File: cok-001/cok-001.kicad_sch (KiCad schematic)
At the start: 72 parts, among them J3209 ATA Power, J3221 ATA0 for BD, U2101 ADT7461A0002RMZR, U2105 TC7WP3125FK, U2108 ICS651MLFT, U6005 NCP511SN33T1G, U6006 NCP511SN18T1, U6009 NCP511SN33T1G, Y2101 24.576MHz

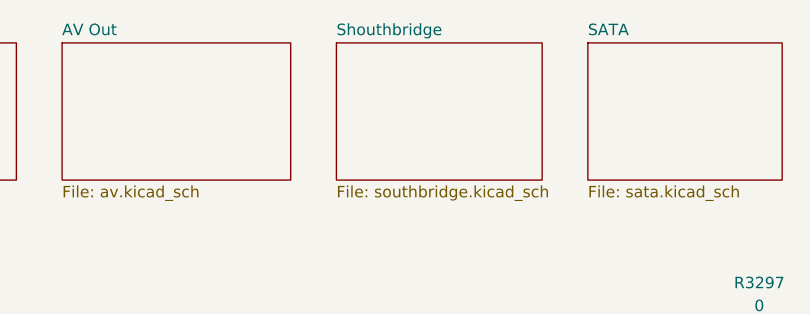
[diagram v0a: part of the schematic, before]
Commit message: L
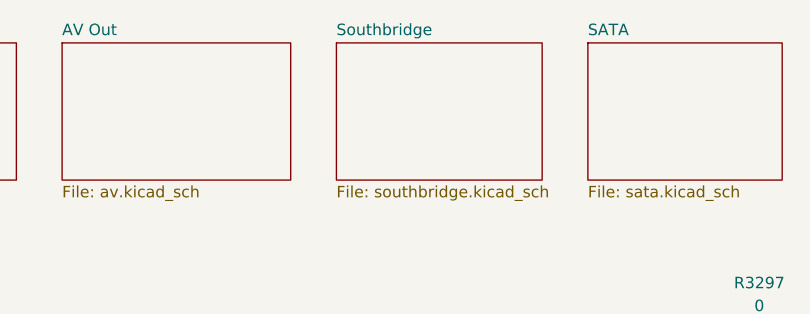
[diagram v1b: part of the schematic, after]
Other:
- sheet Shouthbridge renamed Southbridge
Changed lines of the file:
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@@
 			(color 0 0 0 0.0000)
 		)
-		(property "Sheetname" "Shouthbridge"
+		(property "Sheetname" "Southbridge"
 			(at 364.49 13.2584 0)
 			(effects
@@
 			(project "cok-001"
 				(path "/976eb78d-8215-4cc0-9d72-f9d535c7970b"
-					(page "13")
+					(page "30")
 				)
 			)

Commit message: seperate out
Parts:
- removed C2101, C2102, C2125: XX, Capacitor_SMD:C_0402_1005Metric, symbol Device:C
- removed C2103: 0.001u 50V, Capacitor_SMD:C_0402_1005Metric, symbol Device:C
- removed C2108: 0.1u 10V, Capacitor_SMD:C_0402_1005Metric, symbol Device:C
- removed C2109: 8p, Capacitor_SMD:C_0402_1005Metric, symbol Device:C
- removed C2112: 9p, Capacitor_SMD:C_0402_1005Metric, symbol Device:C
- removed C2271: 0.01u 25V, Capacitor_SMD:C_0402_1005Metric, symbol Device:C
- removed C2272: 100p, Capacitor_SMD:C_0402_1005Metric, symbol Device:C
- removed C3246: 47u 25V, Capacitor_Tantalum_SMD:CP_EIA-3528-15_AVX-H, symbol Device:C_Polarized_US
- removed C3247: 47u 25V, Capacitor_Tantalum_SMD:CP_EIA-7132-28_AVX-C, symbol Device:C_Polarized_US
- removed D3208: LED_Dual_AAKK, Package_TO_SOT_SMD:SC-82AA, symbol Device:LED_Dual_AAKK
- removed F6302: 5A, Fuse:Fuse_1206_3216Metric, symbol Device:Fuse
- removed J3209: ATA Power, Connector_JST:JST_PH_B4B-PH-SM4-TB_1x04-1MP_P2.00mm_Vertical, symbol Connector:Conn_01x04_Socket
- removed J3221: ATA0 for BD, PS3:Hirose_FH12-60S, symbol Connector:Conn_01x60_Pin
- removed L6302: 1uH, Inductor_SMD:L_TDK_SLF6028, symbol Device:L
- removed R2101, R2102: 100, Resistor_SMD:R_0402_1005Metric, symbol Device:R_US
- removed R2103, R2104, R2117: 43,2, Resistor_SMD:R_0402_1005Metric, symbol Device:R_US
- removed R2106: 10k, Resistor_SMD:R_0402_1005Metric, symbol Device:R_US
- removed R2107: 0, Resistor_SMD:R_0603_1608Metric, symbol Device:R_US
- removed R2109: 39, Resistor_SMD:R_0402_1005Metric, symbol Device:R_US
- removed R2123, R2177, R2179: 33, Resistor_SMD:R_0402_1005Metric, symbol Device:R_US
- removed R2181: R, Resistor_SMD:R_0402_1005Metric, symbol Device:R_US
- removed R3211, R3225, R3226, R3227: 0, Resistor_SMD:R_0402_1005Metric, symbol Device:R_US
- removed R3297: 0, Resistor_SMD:R_0805_2012Metric, symbol Device:R_US
- removed U2101: ADT7461A0002RMZR, Package_SO:MSOP-8_3x3mm_P0.65mm, symbol PS3:ADT7461A
- removed U2102: ~, Package_SO:SSOP-24_3.9x8.7mm_P0.635mm, symbol PS3:ICS422A
- removed U2105: TC7WP3125FK, Package_SO:VSSOP-8_2.3x2mm_P0.5mm, symbol PS3:TC7WP3125FK
- removed U2108: ICS651MLFT, Package_SO:SOIC-8_3.9x4.9mm_P1.27mm, symbol PS3:ICS651
- removed Y2101: 24.576MHz, Crystal:Crystal_SMD_5032-2Pin_5.0x3.2mm, symbol Device:Crystal
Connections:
- no-connect marks 3 -> 0
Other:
- added sheet External (external.kicad_sch)
- added sheet RSX Setting (rsxsetting.kicad_sch)
- added sheet SB MISC (sbmisc.kicad_sch)
- added sheet VRM for RSX (rsxvrm.kicad_sch)
- moved on the sheet: C5064, C5070, C5153, C6116, C6117, C6118, C6217, C6218, H1, H10, H11, H12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

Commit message: update to 9
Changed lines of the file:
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@@
 (kicad_sch
-	(version 20231120)
+	(version 20250114)
 	(generator "eeschema")
-	(generator_version "8.0")
+	(generator_version "9.0")
 	(paper "A4")
 	(junction
@@
 		(at 363.22 15.24)
 		(size 25.4 15.24)
+		(exclude_from_sim no)
+		(in_bom yes)
+		(on_board yes)
+		(dnp no)
 		(fields_autoplaced yes)
 		(stroke
@@
 		(at 76.2 15.24)
 		(size 25.4 15.24)
+		(exclude_from_sim no)
+		(in_bom yes)
+		(on_board yes)
+		(dnp no)
 		(fields_autoplaced yes)
 		(stroke
@@
 		(at 15.24 38.1)
 		(size 22.86 15.24)
+		(exclude_from_sim no)
+		(in_bom yes)
+		(on_board yes)
+		(dnp no)
 		(fields_autoplaced yes)
 		(stroke
@@
 		(at 332.74 15.24)
 		(size 25.4 15.24)
+		(exclude_from_sim no)
+		(in_bom yes)
+		(on_board yes)
+		(dnp no)
 		(fields_autoplaced yes)
 		(stroke
@@
 		(at 302.26 38.1)
 		(size 27.94 15.24)
+		(exclude_from_sim no)
+		(in_bom yes)
+		(on_board yes)
+		(dnp no)
 		(fields_autoplaced yes)
 		(stroke
@@
 		(at 110.49 15.24)
 		(size 26.67 15.24)
+		(exclude_from_sim no)
+		(in_bom yes)
+		(on_board yes)
+		(dnp no)
 		(fields_autoplaced yes)
 		(stroke
@@
 		(at 144.78 15.24)
 		(size 25.4 15.24)
+		(exclude_from_sim no)
+		(in_bom yes)
+		(on_board yes)
+		(dnp no)
 		(fields_autoplaced yes)
 		(stroke
@@
 		(at 209.55 15.24)
 		(size 24.13 15.24)
+		(exclude_from_sim no)
+		(in_bom yes)
+		(on_board yes)
+		(dnp no)
 		(fields_autoplaced yes)
 		(stroke
@@
 		(at 177.8 15.24)
 		(size 25.4 15.24)
+		(exclude_from_sim no)
+		(in_bom yes)
+		(on_board yes)
+		(dnp no)
 		(fields_autoplaced yes)
 		(stroke
@@
 		(at 419.1 15.24)
 		(size 25.4 15.24)
+		(exclude_from_sim no)
+		(in_bom yes)
+		(on_board yes)
+		(dnp no)
 		(fields_autoplaced yes)
 		(stroke
@@
 		(at 269.24 15.24)
 		(size 25.4 15.24)
+		(exclude_from_sim no)
+		(in_bom yes)
+		(on_board yes)
+		(dnp no)
 		(fields_autoplaced yes)
 		(stroke
@@
 		(at 238.76 15.24)
 		(size 25.4 15.24)
+		(exclude_from_sim no)
+		(in_bom yes)
+		(on_board yes)
+		(dnp no)
 		(fields_autoplaced yes)
 		(stroke
@@
 		(at 45.72 15.24)
 		(size 22.86 15.24)
+		(exclude_from_sim no)
+		(in_bom yes)
+		(on_board yes)
+		(dnp no)
 		(fields_autoplaced yes)
 		(stroke
@@
 		(at 302.26 15.24)
 		(size 25.4 15.24)
+		(exclude_from_sim no)
+		(in_bom yes)
+		(on_board yes)
+		(dnp no)
 		(fields_autoplaced yes)
 		(stroke
@@
 		(at 332.74 38.1)
 		(size 25.4 15.24)
+		(exclude_from_sim no)
+		(in_bom yes)
+		(on_board yes)
+		(dnp no)
 		(fields_autoplaced yes)
 		(stroke
@@
 		(at 15.24 15.24)
 		(size 22.86 15.24)
+		(exclude_from_sim no)
+		(in_bom yes)
+		(on_board yes)
+		(dnp no)
 		(fields_autoplaced yes)
 		(stroke
@@
 		(at 363.22 38.1)
 		(size 25.4 15.24)
+		(exclude_from_sim no)
+		(in_bom yes)
+		(on_board yes)
+		(dnp no)
 		(fields_autoplaced yes)
 		(stroke
@@
 		(at 391.16 15.24)
 		(size 25.4 15.24)
+		(exclude_from_sim no)
+		(in_bom yes)
+		(on_board yes)
+		(dnp no)
 		(fields_autoplaced yes)
 		(stroke
@@
 		)
 	)
+	(embedded_fonts no)
 )
